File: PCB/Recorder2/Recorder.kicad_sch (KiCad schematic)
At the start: 57 parts, among them J1 Reset, J2 JST-PH-SM4-TB, J3 TC2030-USB-NL-DS, J4 TF_PUSH, J5 USB-C-Socket-H, Q1 CJ2301, SW1 SW_Push_DPDT, U1 ESP32-S3-MINI-1-N4R2, U2 TPS22916CNYFPR, U3 TP4054, U4 ME6211C33M5G-N, U5 ICS-43434, U6 ICS-43434

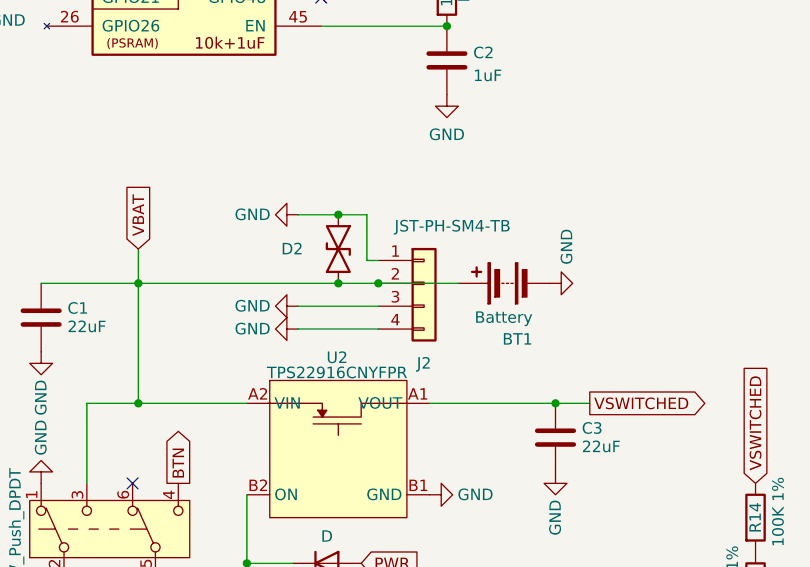
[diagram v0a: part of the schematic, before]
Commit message: Tidy
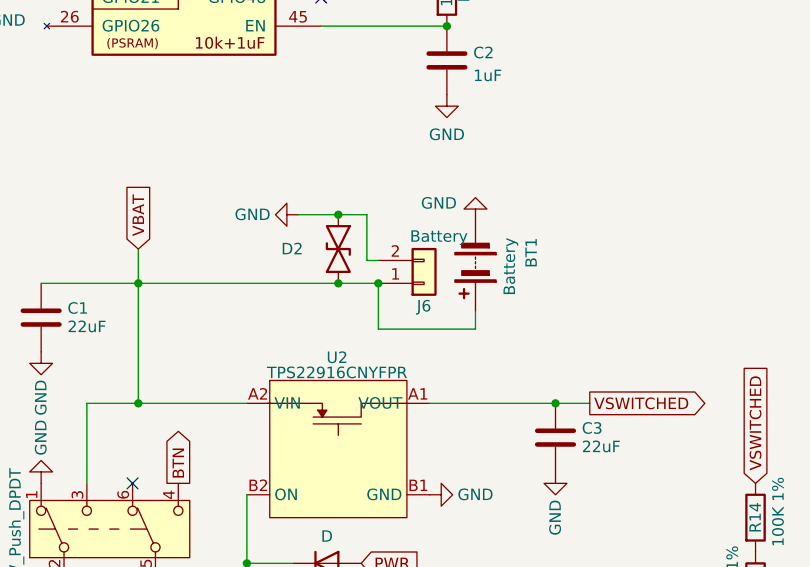
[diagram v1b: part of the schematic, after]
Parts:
- removed J2: JST-PH-SM4-TB, RevK:JST_PH_S2B-PH-SM4-TB_1x02-1MP_P2.00mm_Horizontal, symbol Connector_Generic:Conn_01x04
- added J6: Battery, RevK:1.25T-2PWT (Molex 532610271), symbol Connector_Generic:Conn_01x02
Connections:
- net GND: now also J6.2 (Pin_2)
- net VBAT: now also J6.1 (Pin_1)
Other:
- moved on the sheet: BT1
